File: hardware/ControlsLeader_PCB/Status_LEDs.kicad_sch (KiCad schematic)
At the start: 25 parts, among them J5 BPS_Fault_LED

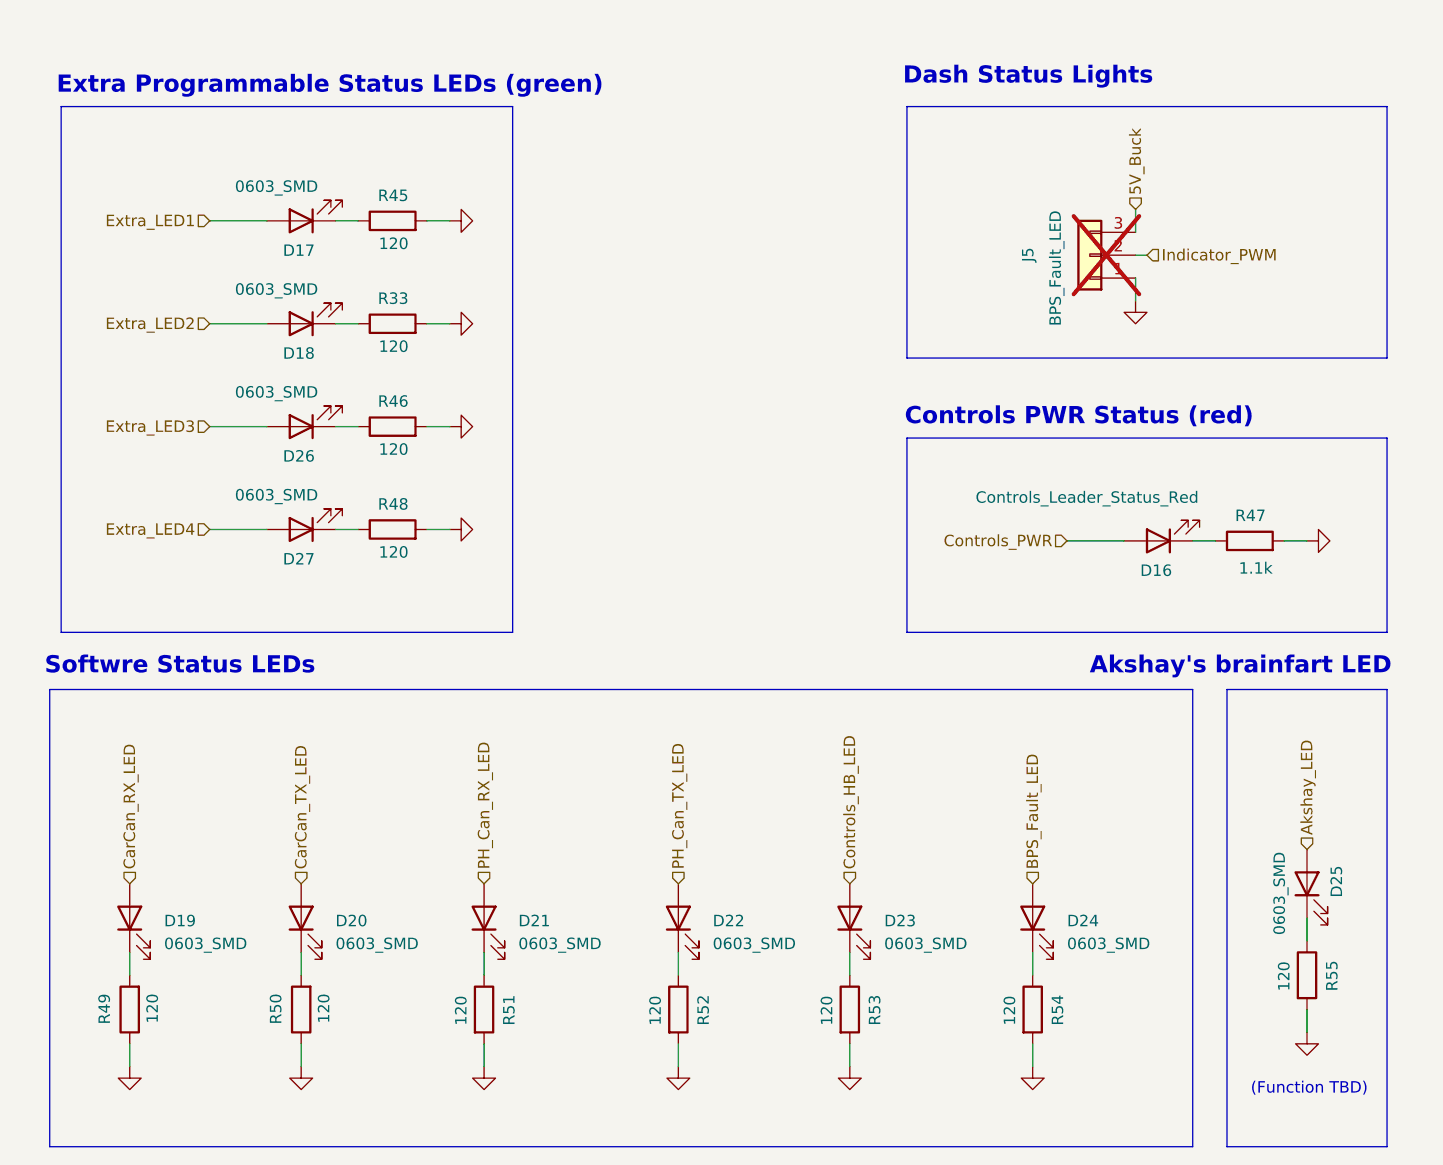
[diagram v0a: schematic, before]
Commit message: revb layout, working on silkscreen
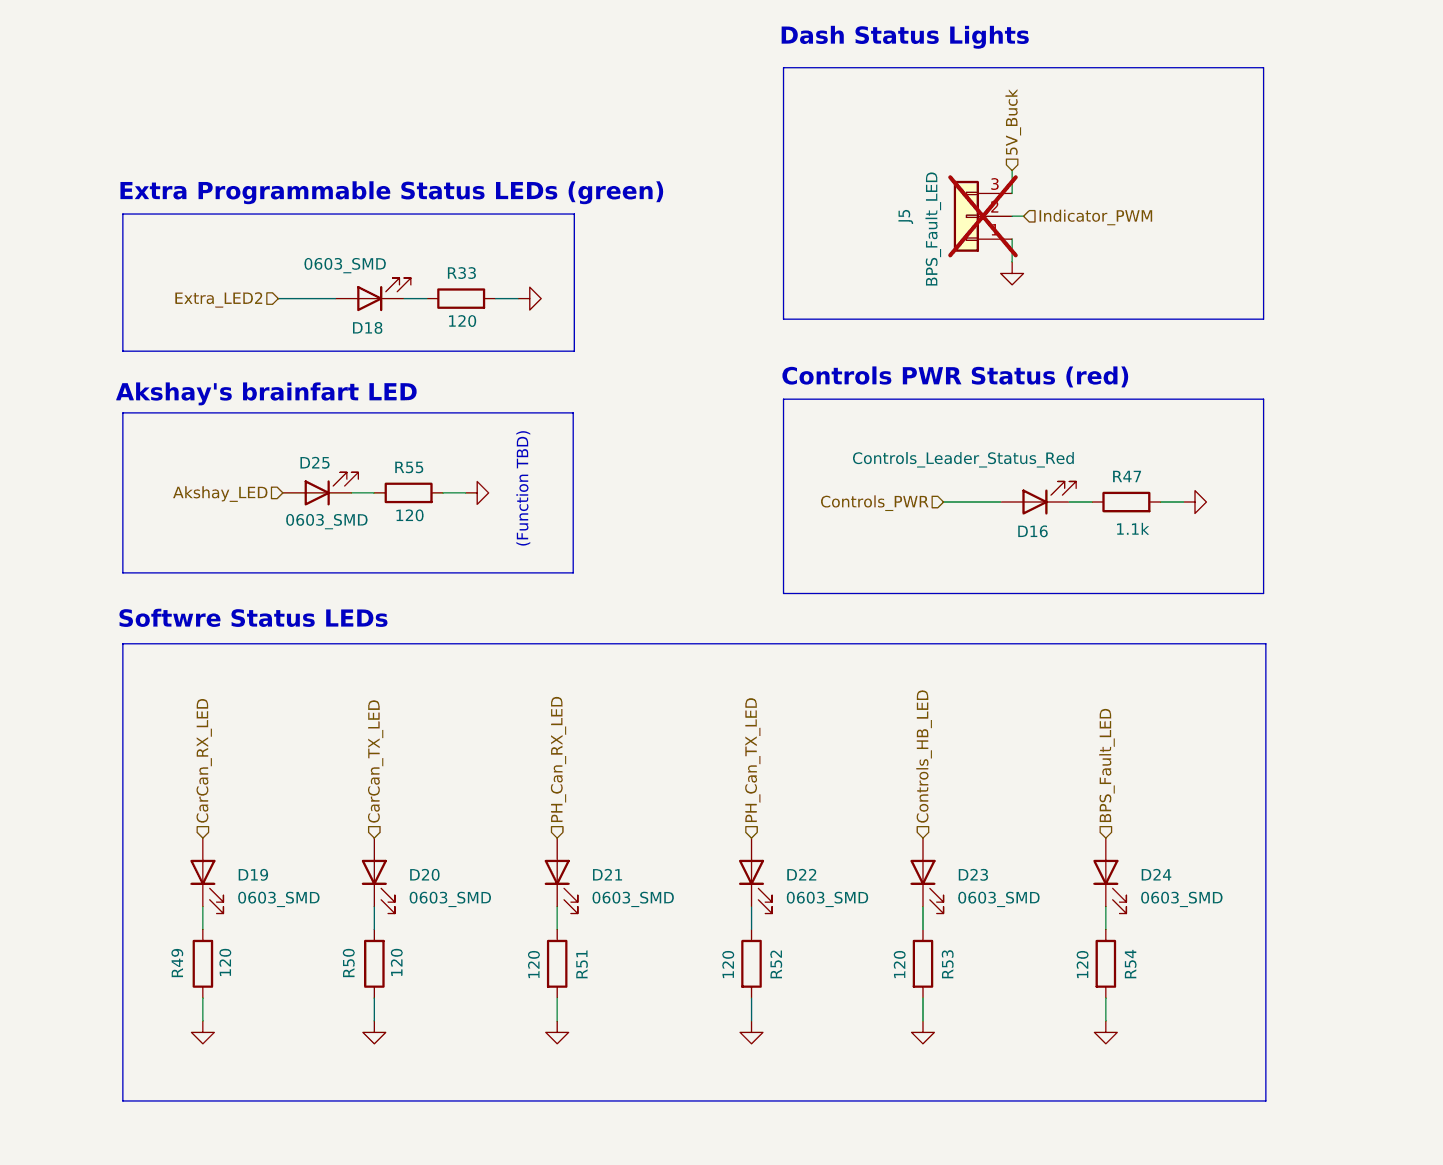
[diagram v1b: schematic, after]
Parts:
- removed D17, D26, D27: 0603_SMD, LED_SMD:LED_0603_1608Metric_Pad1.05x0.95mm_HandSolder, symbol Device:LED
- removed R45, R46, R48: 120, Resistor_SMD:R_0603_1608Metric_Pad0.98x0.95mm_HandSolder, symbol Device:R
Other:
- moved on the sheet: D16, D18, D19, D20, D21, D22, D23, D24, D25, J5, R33, R47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
